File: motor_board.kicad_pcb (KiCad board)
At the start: 2 copper layers, 100 x 80 mm, 28 parts, among them J1 MyRIO_C, J10 Conn_01x05, J11 Barrel_Jack_Switch, J2 BNC, J3 ESCON_24-2, J4 BNC, J5 Conn_01x08, J6 Conn_01x05, J7 Conn_01x05, J8 Conn_01x04, J9 Conn_01x02, SW1 SW_Push, SW2 SW_Push

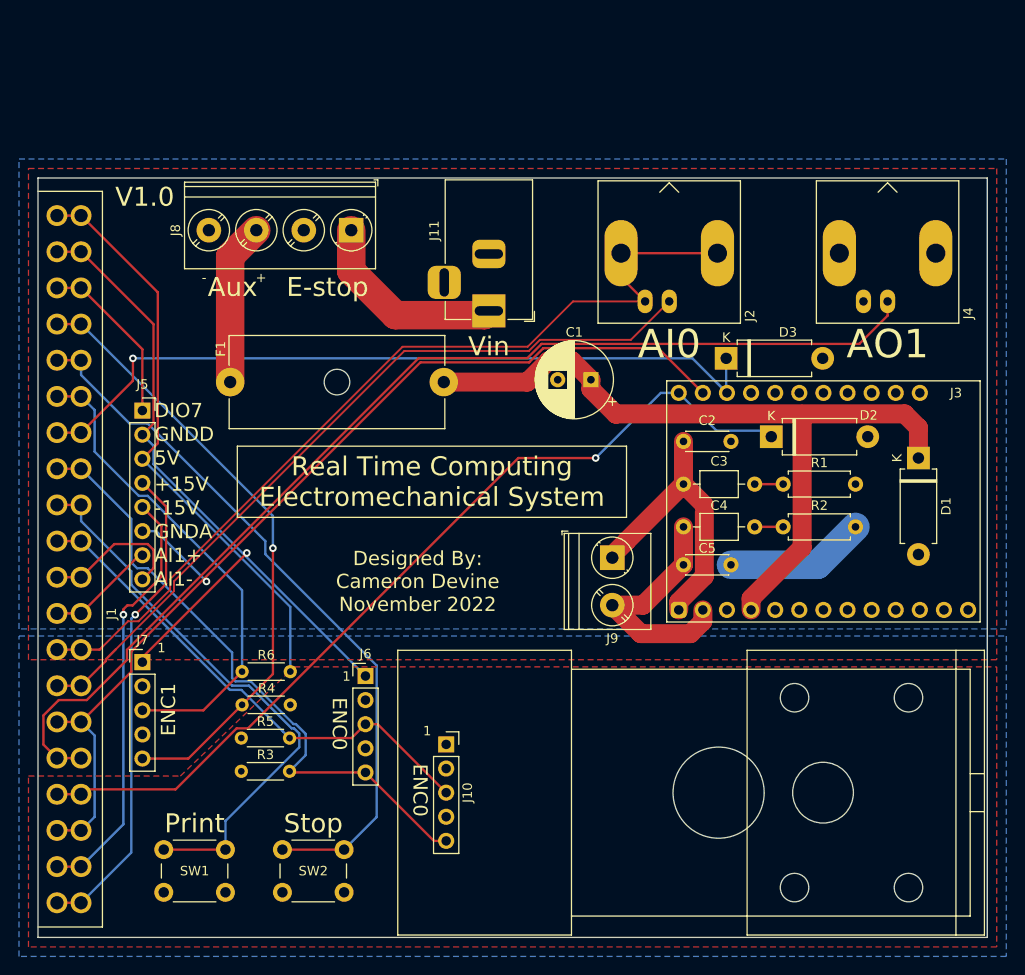
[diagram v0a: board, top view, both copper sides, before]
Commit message: twisted the motor and added a couple connectors
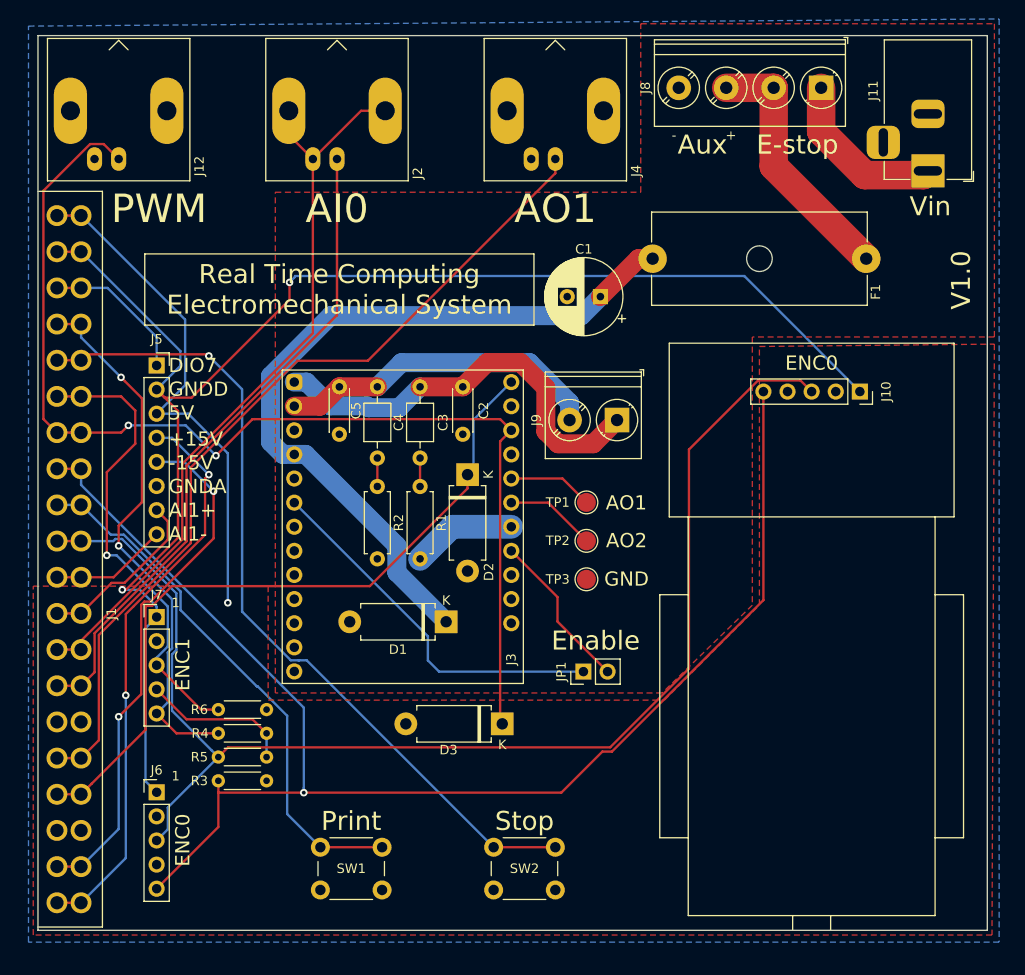
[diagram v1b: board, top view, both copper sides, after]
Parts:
- added J12: BNC, Connector_Coaxial:BNC_Amphenol_B6252HB-NPP3G-50_Horizontal, F.Cu at (46.5, 56.0)
- added JP1: Jumper_2_Bridged, Connector_PinHeader_2.54mm:PinHeader_1x02_P2.54mm_Vertical, F.Cu at (95.5, 110.0)
- added TP1: TestPoint, TestPoint:TestPoint_Pad_D2.0mm, F.Cu at (95.8, 92.2)
- added TP2: TestPoint, TestPoint:TestPoint_Pad_D2.0mm, F.Cu at (95.8, 96.2)
- added TP3: TestPoint, TestPoint:TestPoint_Pad_D2.0mm, F.Cu at (95.8, 100.3)
- moved J10 57.2 mm to (119.5, 80.5), turned to 270 degrees
- moved D1 52.7 mm to (81.0, 104.8), turned to 180 degrees
- moved J8 51.7 mm to (120.5, 48.5)
- moved J11 48.5 mm to (131.8, 57.2)
- moved J3 47.1 mm to (65.0, 79.5), turned to 90 degrees
- moved D3 45.2 mm to (86.9, 115.5), turned to 180 degrees
- moved R2 43.0 mm to (73.8, 90.5), turned to 270 degrees
- moved C5 40.8 mm to (69.8, 80.0), turned to 270 degrees
- moved R1 38.3 mm to (78.2, 90.5), turned to 270 degrees
- moved J2 38.1 mm to (69.5, 56.0)
- moved J4 38.1 mm to (92.5, 56.0)
- moved C4 35.5 mm to (73.8, 80.0), turned to 270 degrees
- moved D2 32.2 mm to (83.2, 89.2), turned to 270 degrees
- moved C3 29.6 mm to (78.2, 80.0), turned to 270 degrees
- moved F1 25.6 mm to (102.8, 66.5), turned to 0 degrees
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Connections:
- J3 pad 17: (no net) -> Net-(J3-Pad17)
- J3 pad 19: (no net) -> Net-(J3-Pad19)
- J3 pad 20: (no net) -> Net-(J3-Pad20)
- J3 pad 6: (no net) -> /+5
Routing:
- net GNDA: track 112.5 -> 0.00 mm, vias 1 -> 0
- net /ENC0.A: track 53.2 -> 138.9 mm
- net /ENC0.B: track 66.2 -> 148.2 mm, vias 0 -> 1
- net GNDD: track 77.0 -> 158.4 mm, vias 1 -> 2
- net /+5: track 0.00 -> 39.3 mm
- net /PWM: track 82.0 -> 120.4 mm, vias 1 -> 2
- net /AO1: track 116.1 -> 90.7 mm
- net /CUR: track 94.7 -> 77.3 mm, vias 1 -> 0
- net Net-(J3-Pad17): track 0.00 -> 16.9 mm
- net /M+: track 29.9 -> 44.4 mm
- net /AI0-: track 94.1 -> 80.2 mm
- net /AI0+: track 82.0 -> 69.2 mm
- net /BUT2: track 76.0 -> 88.1 mm, vias 0 -> 1
- net /-15V: track 45.1 -> 55.5 mm, vias 1 -> 2
- net VBUS: track 17.1 -> 27.0 mm
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- added copper zone on F.Cu, net 5V
- removed copper zone on B.Cu, net 5V
- removed copper zone on F.Cu, net GNDD
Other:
- board size 100 x 80 mm -> 100 x 94.2 mm
- net class Input Power: trace_width 3 -> 2.5
- board text added: "AO2"
- board text added: "Enable"
- board text added: "GND"
- board text added: "PWM"
